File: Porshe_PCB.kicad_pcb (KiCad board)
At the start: 2 copper layers, 80 x 80 mm, 54 parts, among them IC2 BH1750FVI-TR, J1 TF-115, J10 Conn_01x01_Pin, J11 Conn_01x01_Pin, J12 Conn_01x01_Pin, J13 Barrel_Jack, J14 Conn_02x20_Odd_Even, J15 Conn_01x03_Pin, J16 Conn_02x20_Odd_Even, J17 Conn_01x03_Pin, J18 Conn_01x01_Pin, J19 Conn_01x01_Pin, J2 SM04B-SRSS-TB_LF__SN_, J3 Conn_02x02_Odd_Even, J4 S2B-PH-SM4-TB_LF__SN_, J5 Conn_01x01_Pin, J6 Conn_01x01_Pin, J7 Conn_01x01_Pin, J8 Conn_01x01_Pin, J9 Conn_02x04_Odd_Even, Q1 DMG2305UX-7, Q2 2N3904, U1 DS3231SN

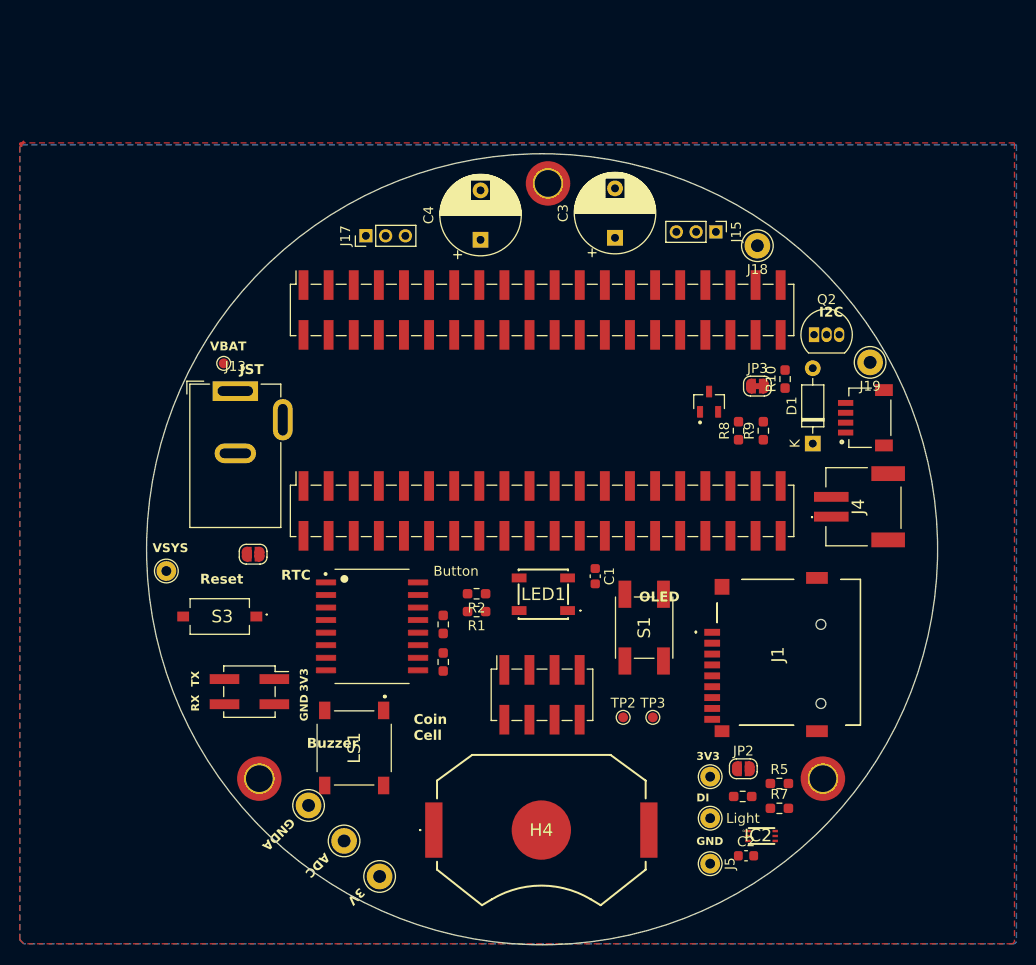
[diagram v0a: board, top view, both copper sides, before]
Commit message: 첫번째 완성
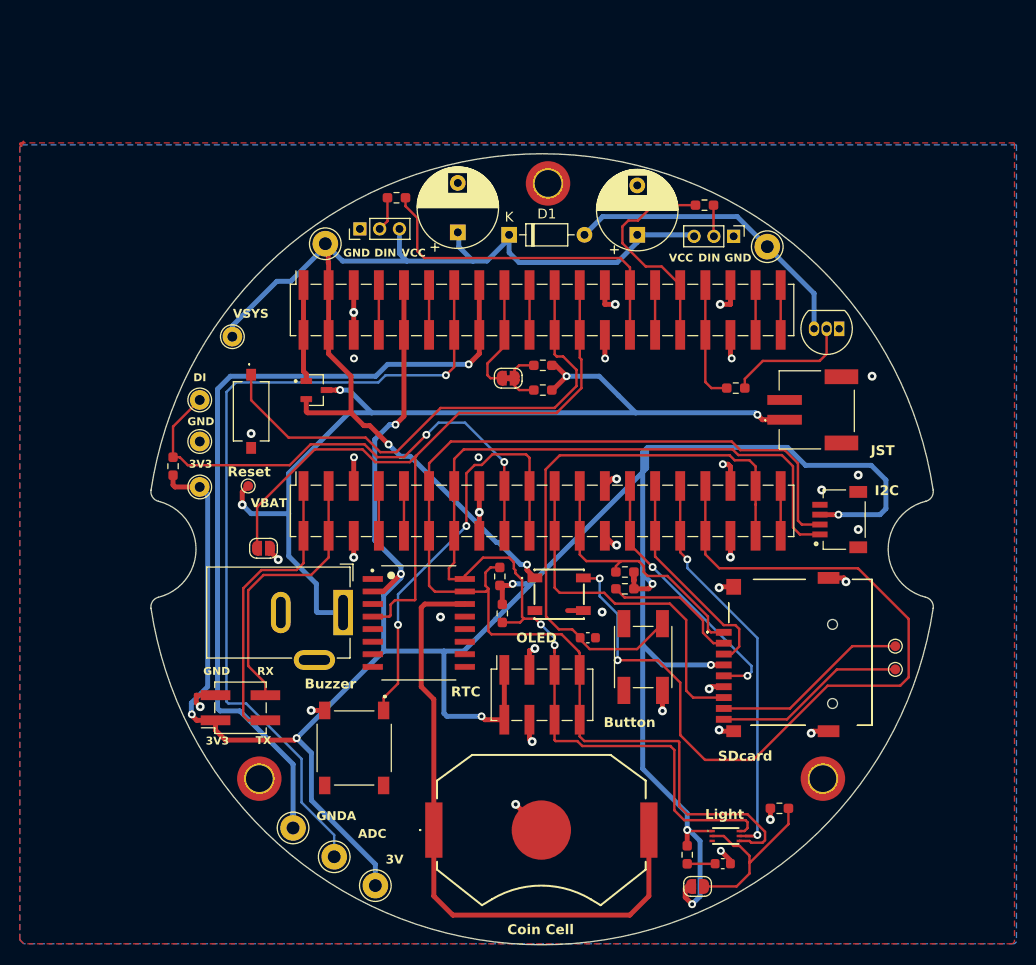
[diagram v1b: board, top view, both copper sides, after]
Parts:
- added G***: LOGO, SmartFarm:DataPi_gondo, B.Cu at (132.6, 106.1)
- added R11: 220, Resistor_SMD:R_0603_1608Metric_Pad0.98x0.95mm_HandSolder, F.Cu at (149.1, 63.7)
- added R12: 220, Resistor_SMD:R_0603_1608Metric_Pad0.98x0.95mm_HandSolder, F.Cu at (117.9, 63.0)
- moved R6 66.6 mm to (95.3, 90.1), turned to -90 degrees
- moved J11 64.2 mm to (98.0, 87.6)
- moved J5 64.2 mm to (98.0, 92.2)
- moved J10 64.2 mm to (98.0, 83.4)
- moved J18 43.7 mm to (110.7, 67.6)
- moved Q1 39.7 mm to (109.8, 82.4), turned to 0 degrees
- moved D1 37.3 mm to (129.3, 66.7), turned to 0 degrees
- moved TP2 28.5 mm to (168.3, 108.3), turned to -90 degrees
- moved JP3 25.2 mm to (129.2, 81.2), turned to 180 degrees
- moved TP3 25.0 mm to (168.3, 110.7), turned to -90 degrees
- moved J13 24.9 mm to (112.5, 104.9), turned to -90 degrees
- moved J12 24.6 mm to (101.3, 77.0)
- moved R9 23.3 mm to (132.7, 79.9), turned to 0 degrees
- moved S3 21.0 mm to (103.2, 84.5), turned to -90 degrees
- moved R8 20.2 mm to (132.7, 82.4), turned to 0 degrees
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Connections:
- net /SPI0_MISO renamed /SPI1_MISO
- net /SPI0_MOSI renamed /SPI1_MOSI
- net /SPI_SC renamed /SPI1_SC
- C3 pad 1: Net-(J15-Pin_3) -> /VSYS
- C4 pad 1: Net-(J17-Pin_3) -> /VSYS
- J1 pad 5: /SPI0_SCK -> /SPI1_SCK
- J15 pad 1: /3V3 -> GND
- J15 pad 2: /DIN_1 -> Net-(J15-Pin_2)
- J15 pad 3: Net-(J15-Pin_3) -> /VSYS
- J17 pad 1: /3V3 -> GND
- J17 pad 2: /DIN_2 -> Net-(J17-Pin_2)
- J17 pad 3: Net-(J17-Pin_3) -> /VSYS
- LED1 pad 1: /3V3 -> /VSYS
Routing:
- net /3V3: track 0.00 -> 282.0 mm, vias 0 -> 11
- net /SDA: track 0.00 -> 122.9 mm
- net /SCL: track 0.00 -> 116.4 mm, vias 0 -> 2
- net /VSYS: track 0.00 -> 113.8 mm, vias 0 -> 2
- net /VBAT(+): track 0.00 -> 96.6 mm, vias 0 -> 4
- net /LED: track 0.00 -> 87.0 mm, vias 0 -> 2
- net GNDA: track 0.00 -> 85.2 mm, vias 0 -> 1
- net /ADC2: track 0.00 -> 84.9 mm, vias 0 -> 1
- net /RTC_RST: track 0.00 -> 73.8 mm
- net /BAK_VBAT: track 0.00 -> 64.3 mm
- net GND: track 0.00 -> 63.9 mm, vias 0 -> 35
- net /SW1: track 0.00 -> 58.6 mm
- net /DI: track 0.00 -> 53.5 mm, vias 0 -> 2
- net /RUN: track 0.00 -> 51.9 mm
- net /Buzz: track 0.00 -> 42.7 mm, vias 0 -> 2
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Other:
- board size 80 x 80 mm -> 79.1 x 80 mm
- board text added: "DIN"
- board text added: "SDcard"
- board text added: "VCC"

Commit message: 오토라우딩하기전
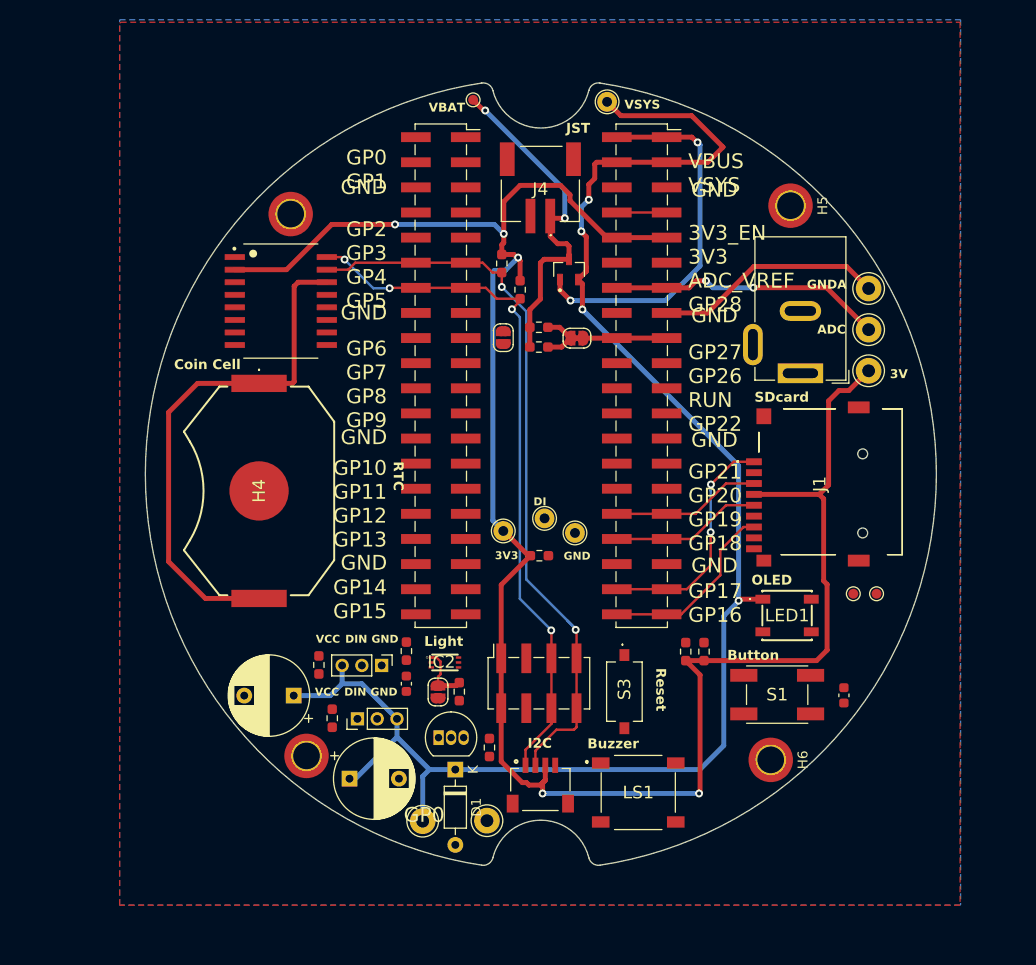
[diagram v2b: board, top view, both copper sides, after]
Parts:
- removed H1: MountingHole_Pad, MountingHole:MountingHole_2.7mm_M2.5_ISO7380_Pad_TopOnly
- removed J3: Conn_02x02_Odd_Even, Connector_PinSocket_2.54mm:PinSocket_2x02_P2.54mm_Vertical_SMD
- added H5: MountingHole_Pad, MountingHole:MountingHole_2.7mm_M2.5_ISO7380_Pad_TopOnly, F.Cu at (157.8, 63.8)
- added H6: MountingHole_Pad, MountingHole:MountingHole_2.7mm_M2.5_ISO7380_Pad_TopOnly, F.Cu at (155.8, 119.8)
- moved J7 79.8 mm to (165.7, 72.1), turned to -35 degrees
- moved J6 75.9 mm to (165.7, 76.3), turned to -35 degrees
- moved J8 72.1 mm to (165.7, 80.5), turned to -35 degrees
- moved J19 64.6 mm to (127.0, 126.0)
- moved C3 62.2 mm to (113.1, 121.7), turned to 0 degrees
- moved R11 60.7 mm to (110.0, 110.2), turned to -90 degrees
- moved J18 59.2 mm to (120.5, 126.0)
- moved Q2 57.9 mm to (122.2, 117.5), turned to 0 degrees
- moved H2 57.2 mm to (107.2, 64.6), turned to -90 degrees
- moved J15 56.1 mm to (116.4, 110.2)
- moved D1 54.4 mm to (123.8, 120.8), turned to -90 degrees
- moved R12 53.0 mm to (111.4, 115.6), turned to 90 degrees
- moved H3 52.3 mm to (108.8, 119.4), turned to -90 degrees
- moved J13 52.2 mm to (158.8, 80.7), turned to 180 degrees
- moved C4 49.7 mm to (107.5, 113.3), turned to 180 degrees
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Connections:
- J1 pad 1: /SPI1_SC -> /SPI0_SC
- J1 pad 3: /SPI1_MOSI -> /SPI0_MOSI
- J1 pad 5: /SPI1_SCK -> /SPI0_SCK
- J1 pad 7: /SPI1_MISO -> /SPI0_MISO
- J14 pad 19: Net-(J14-Pin_19) -> /DI
- J14 pad 20: Net-(J14-Pin_19) -> /DI
- J14 pad 23: /RTC_RST -> /Buzz
- J14 pad 24: /RTC_RST -> /Buzz
- J14 pad 27: /DIN_2 -> /LED
- J14 pad 28: /DIN_2 -> /LED
- J14 pad 29: Net-(J14-Pin_29) -> /SW1
- J14 pad 30: Net-(J14-Pin_29) -> /SW1
- J14 pad 31: /DIN_1 -> /SPI0_MOSI
- J14 pad 32: /DIN_1 -> /SPI0_MOSI
- J14 pad 33: /FAN -> /SPI0_SCK
- J14 pad 34: /FAN -> /SPI0_SCK
- J14 pad 37: Net-(J14-Pin_37) -> /SPI0_SC
- J14 pad 38: Net-(J14-Pin_37) -> /SPI0_SC
- J14 pad 39: Net-(J14-Pin_39) -> /SPI0_MISO
- J14 pad 40: Net-(J14-Pin_39) -> /SPI0_MISO
- J16 pad 19: /Buzz -> /RTC_RST
- J16 pad 20: /Buzz -> /RTC_RST
- J16 pad 21: /SPI1_MISO -> Net-(J16-Pin_21)
- J16 pad 22: /SPI1_MISO -> Net-(J16-Pin_21)
- J16 pad 23: /SPI1_SC -> Net-(J16-Pin_23)
- J16 pad 24: /SPI1_SC -> Net-(J16-Pin_23)
- J16 pad 27: /SPI1_SCK -> Net-(J16-Pin_27)
- J16 pad 28: /SPI1_SCK -> Net-(J16-Pin_27)
- J16 pad 29: /SPI1_MOSI -> Net-(J16-Pin_29)
- J16 pad 30: /SPI1_MOSI -> Net-(J16-Pin_29)
- J16 pad 33: /LED -> /FAN
- J16 pad 34: /LED -> /FAN
- J16 pad 37: /SW1 -> /DIN_1
- J16 pad 38: /SW1 -> /DIN_1
- J16 pad 39: Net-(J16-Pin_39) -> /DIN_2
- J16 pad 40: Net-(J16-Pin_39) -> /DIN_2
- R2 pad 1: /SPI1_SC -> /SPI0_SC
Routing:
- net /LED: track 87.0 -> 0.00 mm, vias 2 -> 0
- net /RTC_RST: track 73.8 -> 0.00 mm
- net /3V3: track 282.0 -> 211.4 mm, vias 11 -> 5
- net GND: track 63.9 -> 0.00 mm, vias 35 -> 0
- net GNDA: track 85.2 -> 23.3 mm, vias 1 -> 0
- net /VBAT(+): track 96.6 -> 35.2 mm, vias 4 -> 2
- net /SW1: track 58.6 -> 0.00 mm
- net /ADC2: track 84.9 -> 27.8 mm, vias 1 -> 2
- net /DI: track 53.5 -> 0.00 mm, vias 2 -> 0
- net /RUN: track 51.9 -> 0.00 mm
- net /SDA: track 122.9 -> 75.3 mm, vias 0 -> 2
- net /VSYS: track 113.8 -> 161.1 mm, vias 2 -> 4
- net /SCL: track 116.4 -> 71.8 mm, vias 2 -> 4
- net /Buzz: track 42.7 -> 0.00 mm, vias 2 -> 0
- net /Light_RST: track 41.5 -> 0.00 mm, vias 2 -> 0
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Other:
- board size 79.1 x 80 mm -> 80 x 79.1 mm
- board text added: "GP0"
- board text added: "GP0 GP1 GP2 GP3 GP4 GP5 GP6 GP7 GP8 GP9 GP10 GP11 GP12 GP13 GP14 GP15"
- board text added: "VBUS VSYS 3V3_EN 3V3 ADC_VREF GP28 GP27 GP26 RUN GP22 GP21 GP20 GP19 GP18 GP17 GP16"
- board text removed: "RX"
- board text removed: "TX"
